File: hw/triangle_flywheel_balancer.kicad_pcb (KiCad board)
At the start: 4 copper layers, 55 x 40 mm, 64 parts, among them J1 TYPE-C-31-M-12, J2 BATTERY, J3 MOTOR, J4 SERVO, J5 LATCH, J6 OPEN, J7 CLOSED, Q1 FS8205A, U1 ESP32-C3-MINI-1-N4, U2 DRV8876PWPR, U3 TLV7041DCKR, U4 MCP73831T-2ACI/OT, U5 DW01A, U6 XC6220B331MR-G, U7 TPS61023DRLR

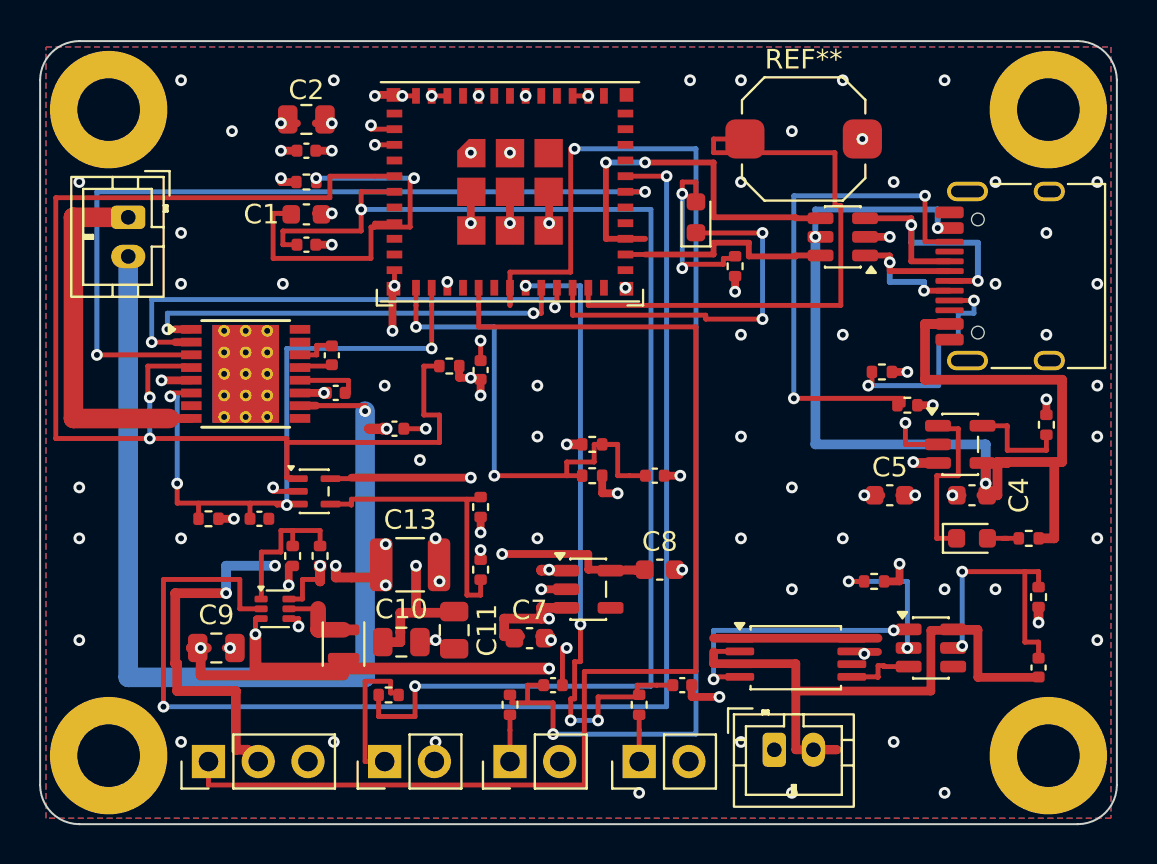
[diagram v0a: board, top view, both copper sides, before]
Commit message: Upd
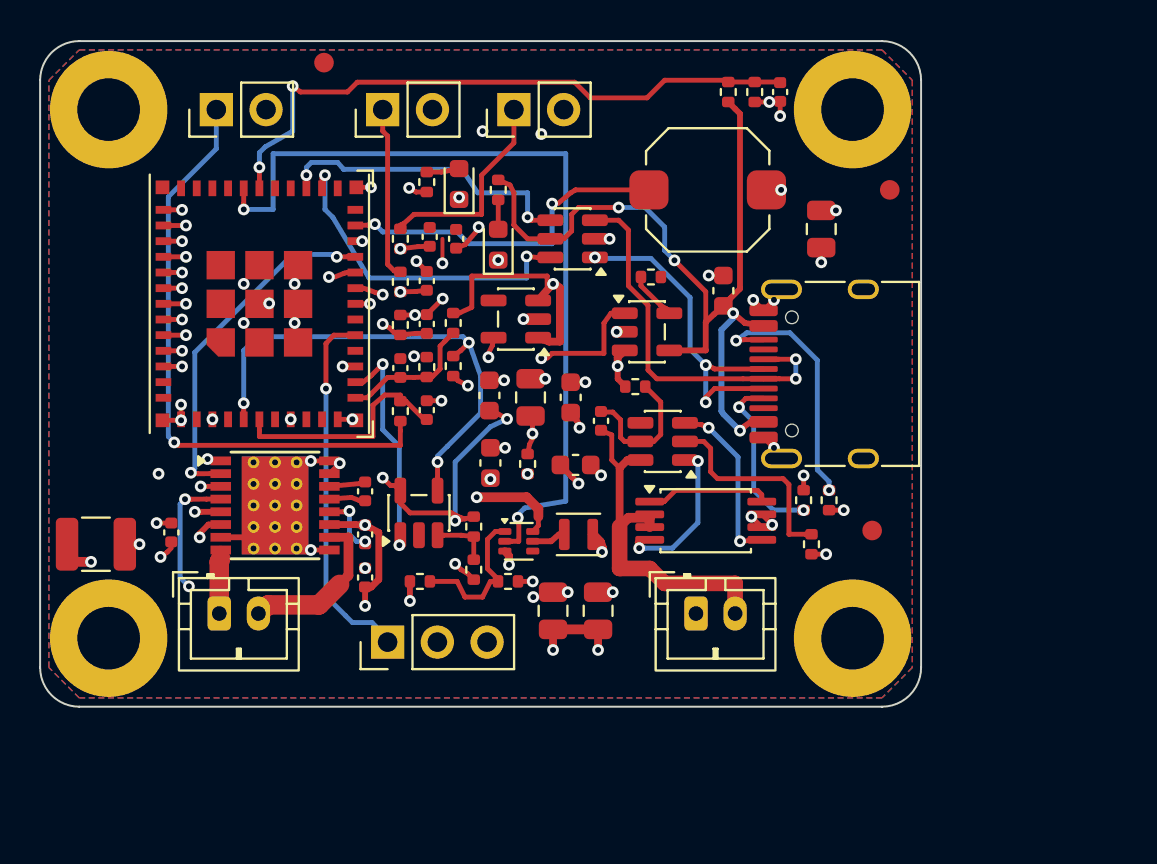
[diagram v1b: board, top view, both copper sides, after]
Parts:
- added C22: 100nF, triangle_flywheel_balancer:C_0402_1005Metric, F.Cu at (137.8, 102.6)
- added FID1: Fiducial, triangle_flywheel_balancer:Fiducial_1mm_Mask2mm, F.Cu at (114.5, 101.1)
- added FID2: Fiducial, triangle_flywheel_balancer:Fiducial_1mm_Mask2mm, F.Cu at (143.4, 107.6)
- added FID3: Fiducial, triangle_flywheel_balancer:Fiducial_1mm_Mask2mm, F.Cu at (142.5, 125.0)
- added R20: 68k, triangle_flywheel_balancer:R_0402_1005Metric, F.Cu at (135.2, 102.6)
- added R21: 100k, triangle_flywheel_balancer:R_0402_1005Metric, F.Cu at (136.5, 102.6)
- R8: value 1.1M -> 110k
- R9: value 150k -> 15k
- U3: value TLV7041DCKR -> TLV1701AIDBVR; footprint triangle_flywheel_balancer:SOT-353_SC-70-5 -> triangle_flywheel_balancer:SOT-23-5
- moved C9 37.6 mm to (139.9, 109.6), turned to 90 degrees
- moved J5 34.4 mm to (109.0, 103.5)
- moved J6 33.9 mm to (117.5, 103.5)
- moved J7 33.9 mm to (124.2, 103.5)
- moved R4 32.4 mm to (123.4, 107.6), turned to -90 degrees
- moved D2 28.5 mm to (123.4, 110.4), turned to 90 degrees
- moved R19 26.7 mm to (118.4, 110.1), turned to -90 degrees
- moved C21 26.3 mm to (119.9, 110.0), turned to 90 degrees
- moved C6 25.7 mm to (128.7, 119.4)
- moved R6 23.2 mm to (130.4, 117.7), turned to 0 degrees
- moved R18 22.3 mm to (118.4, 112.3), turned to -90 degrees
- moved C20 21.6 mm to (119.8, 112.2), turned to 90 degrees
- moved R5 21.6 mm to (131.2, 112.0), turned to 0 degrees
- moved J3 20.8 mm to (109.2, 129.2), turned to 0 degrees
- moved R1 18.3 mm to (124.9, 121.6), turned to -90 degrees
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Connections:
- U1 pad 30: DRV_NSLEEP -> VBUS_DET
- U2 pad 3: DRV_NSLEEP -> +3V3
- U3 pad 1: nFAULT_ANY -> IPROPI
- U3 pad 3: IPROPI -> VTH
- U3 pad 4: VTH -> nFAULT_ANY
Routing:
- net SW_OPEN: track 61.5 -> 4.43 mm
- net SW_LATCH: track 64.8 -> 11.9 mm, vias 2 -> 0
- net SERVO_PWM: track 62.6 -> 18.8 mm, vias 0 -> 1
- net MOTOR_B: track 50.8 -> 8.32 mm, vias 1 -> 0
- net DRV_NSLEEP: track 42.1 -> 0.00 mm, vias 2 -> 0
- net VBUS_DET: track 0.00 -> 32.1 mm, vias 0 -> 2
- net SW_CLOSED: track 32.9 -> 5.64 mm, vias 4 -> 2
- net BOOST_EN: track 67.9 -> 42.8 mm
- net SW_LATCH_J: track 7.51 -> 31.0 mm, vias 0 -> 1
- net VBAT_SENSE: track 26.1 -> 7.05 mm, vias 2 -> 0
- net +5V: track 37.7 -> 20.0 mm, vias 9 -> 7
- net VBUS: track 60.4 -> 43.7 mm, vias 3 -> 4
- net BATT_N: track 34.5 -> 18.5 mm
- net MOTOR_A: track 19.1 -> 3.26 mm
- net nFAULT_ANY: track 64.5 -> 49.3 mm, vias 2 -> 5
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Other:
- board size 55 x 40 mm -> 45 x 34 mm
